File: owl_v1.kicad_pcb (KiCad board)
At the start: 4 copper layers, 39.5 x 73.5 mm, 63 parts, among them J1 USB_C_Receptacle_USB2.0_16P, J10 JST-PH Battery, J3 Screw_Terminal_01x03, J4 SPI1_IMU, J5 I2C, J6 Micro_SD_Card_Det_Hirose_DM3AT, J7 I2C OLED, J8 External GPIOs, SW1 SW_SPDT, U1 STM32F103C8T6, U3 FT230XS, U4 SN65HVD230, U5 TLV73333PDBV, Y1 8MHz, Y2 32k768

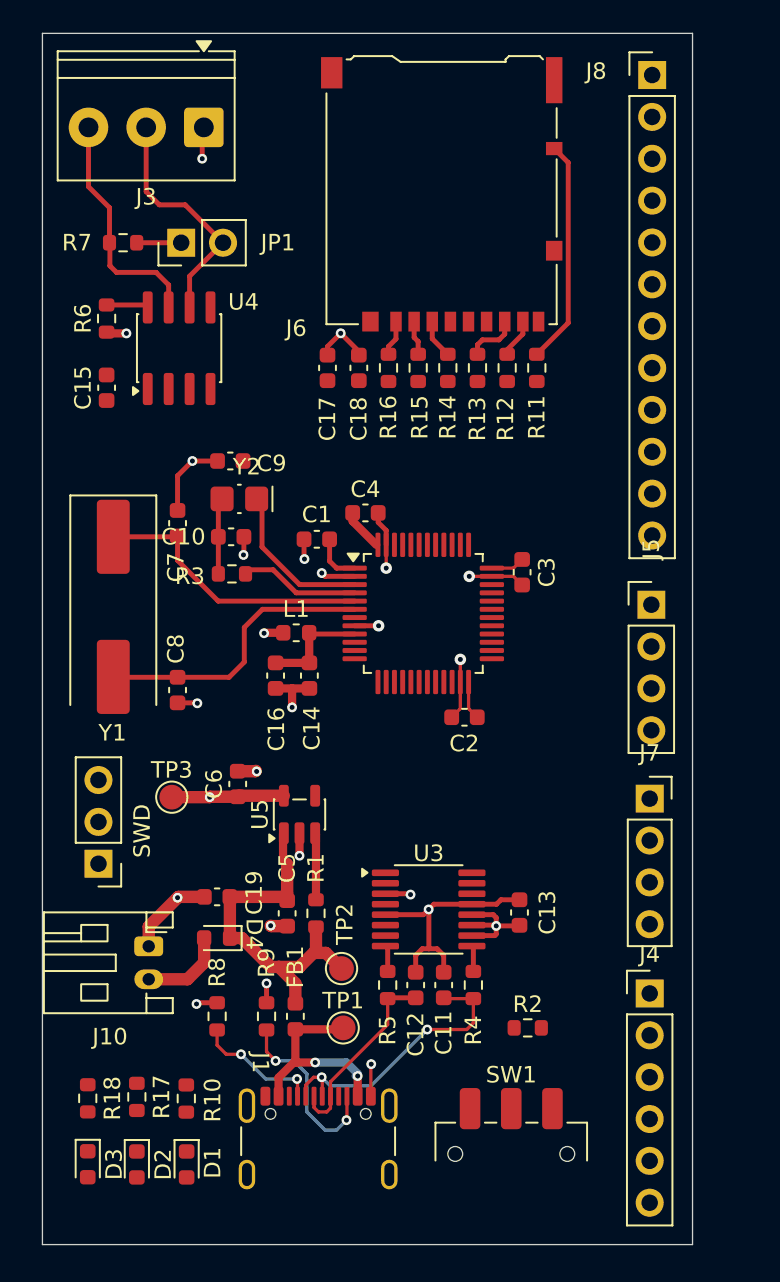
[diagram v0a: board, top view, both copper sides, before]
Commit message: [feat] Finished routing for uSD card reader
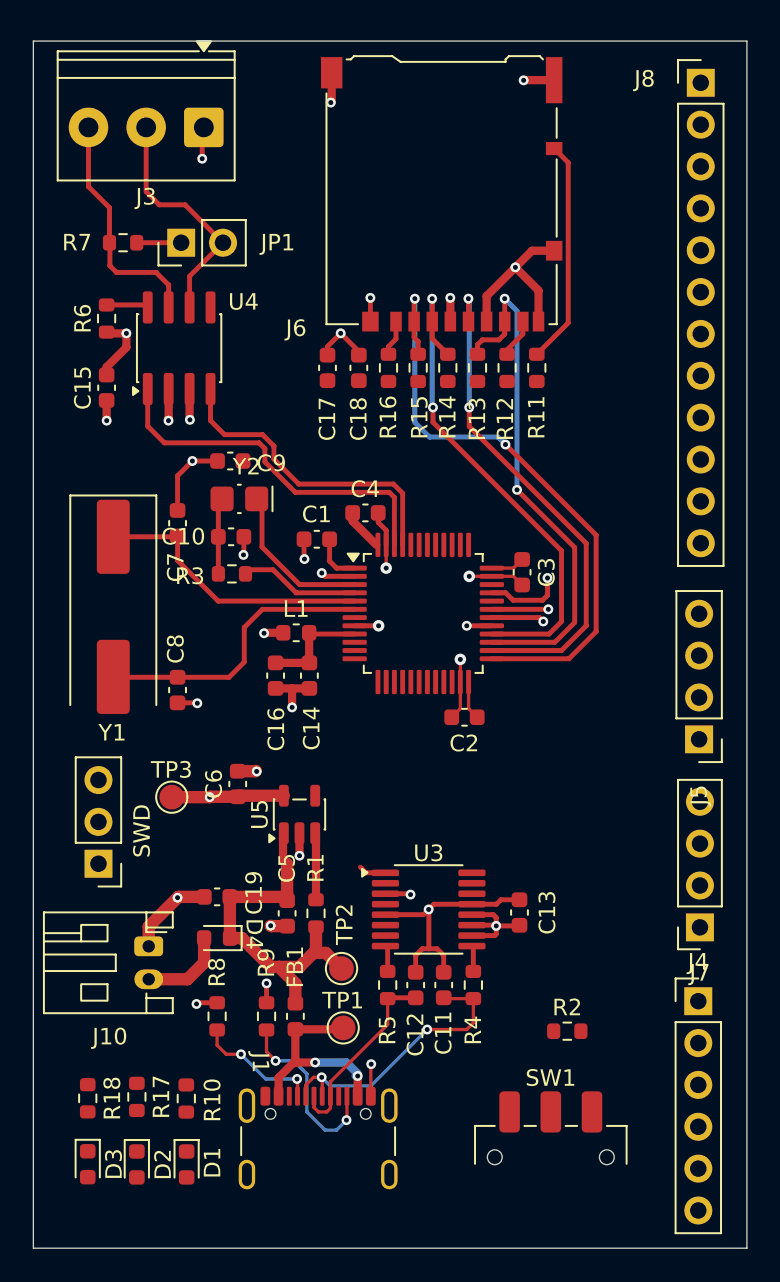
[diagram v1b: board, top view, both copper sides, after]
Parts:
- moved J5 8.67 mm to (191.4, 89.1), turned to 180 degrees
- moved J7 8.38 mm to (191.5, 100.5), turned to 180 degrees
- moved J4 2.99 mm to (191.4, 105.0)
- moved J8 2.99 mm to (191.6, 49.3)
- moved SW1 2.41 mm to (182.4, 114.5)
- moved R2 2.41 mm to (183.4, 106.8)
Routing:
- net SD_CS: track 2.09 -> 37.7 mm, vias 0 -> 2
- net SD_SCK: track 0.00 -> 30.6 mm, vias 0 -> 2
- net SD_MOSI: track 2.38 -> 31.2 mm, vias 0 -> 2
- net SD_MISO: track 3.26 -> 31.6 mm, vias 0 -> 2
- net CAN_TX: track 0.00 -> 22.4 mm
- net GND: track 59.0 -> 79.6 mm, vias 21 -> 26
- net CAN_RX: track 0.00 -> 19.0 mm
- net /owl_v1/USB to UART Bridge/FT230_TXD: track 0.00 -> 5.08 mm, vias 0 -> 1
- net GPIO_6: track 0.00 -> 4.74 mm, vias 0 -> 1
- net +3.3V: track 26.5 -> 31.0 mm, vias 4 -> 7
- net /owl_v1/USB to UART Bridge/FT230_RXD: track 0.00 -> 3.22 mm, vias 0 -> 1
- net GPIO_4: track 0.00 -> 1.52 mm, vias 0 -> 1
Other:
- board size 39.5 x 73.5 mm -> 43.3 x 73.2 mm
